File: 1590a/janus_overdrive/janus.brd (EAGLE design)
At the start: 33 x 33 mm, 27 parts, among them IC1 LM741

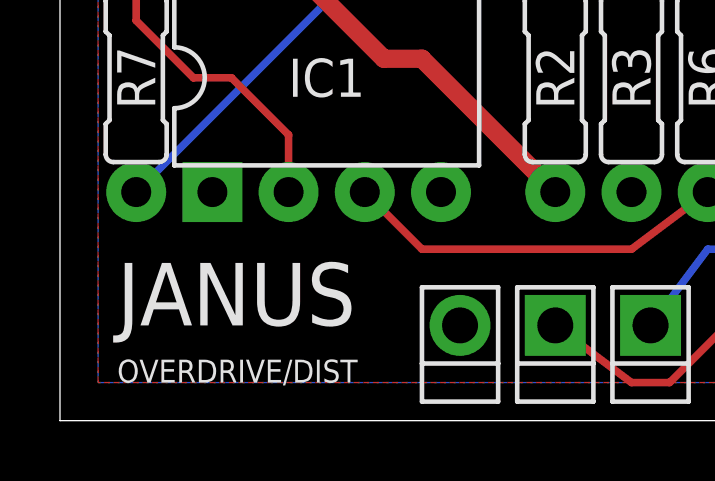
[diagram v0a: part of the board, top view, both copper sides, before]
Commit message: little edits & cleanup
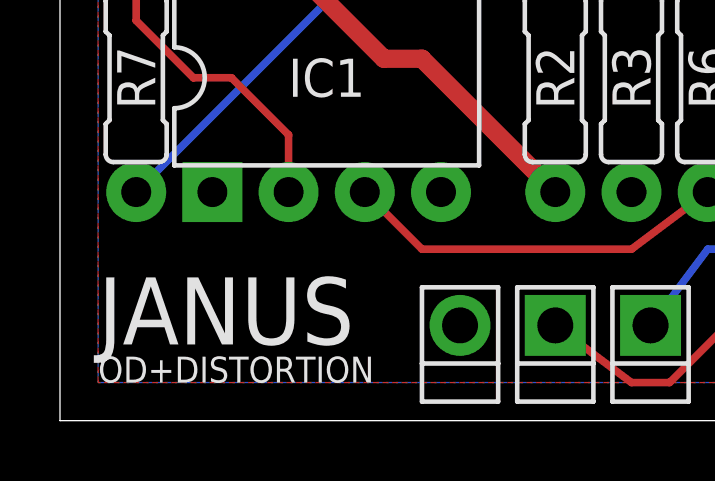
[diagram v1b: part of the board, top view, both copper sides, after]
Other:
- board text added: "OD+DISTORTION"
- board text removed: "OVERDRIVE/DIST"
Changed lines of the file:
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@@
 <text x="22.86" y="1.27" size="0.8128" layer="25" font="vector">burr settles</text>
 <text x="26.67" y="14.605" size="0.8128" layer="25" font="vector">(c)2016</text>
-<text x="1.905" y="1.27" size="0.762" layer="25" font="vector">OVERDRIVE/DIST</text>
-<text x="1.905" y="3.175" size="2.0828" layer="25" font="vector">JANUS</text>
+<text x="1.27" y="1.27" size="0.8636" layer="25" font="vector">OD+DISTORTION</text>
+<text x="1.27" y="2.54" size="2.2352" layer="25" font="vector">JANUS</text>
 </plain>
 <attributes>
